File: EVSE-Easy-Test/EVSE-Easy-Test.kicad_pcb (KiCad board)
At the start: 2 copper layers, 70.1 x 40.9 mm, 17 parts, among them J1 Type 2, J2 CP diag, SW1 PP current, SW2 CP state

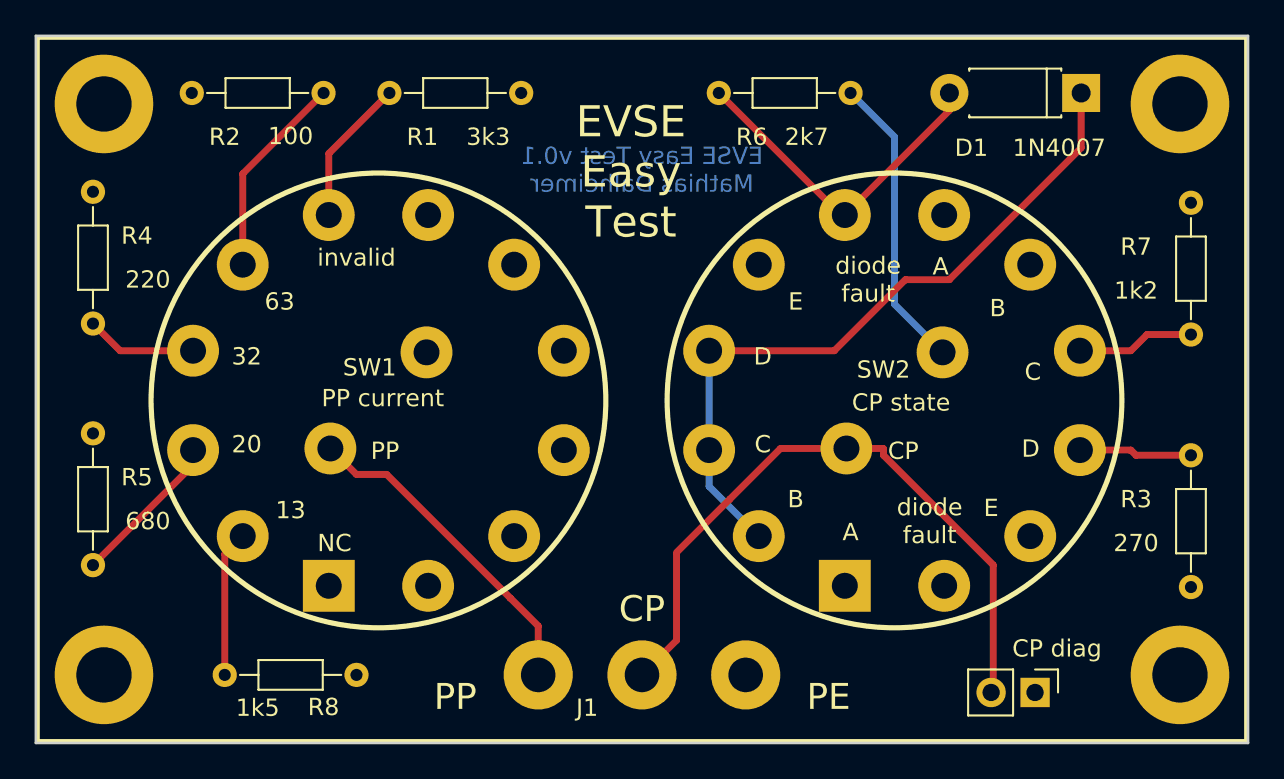
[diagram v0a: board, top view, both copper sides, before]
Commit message: second prototype as ordered
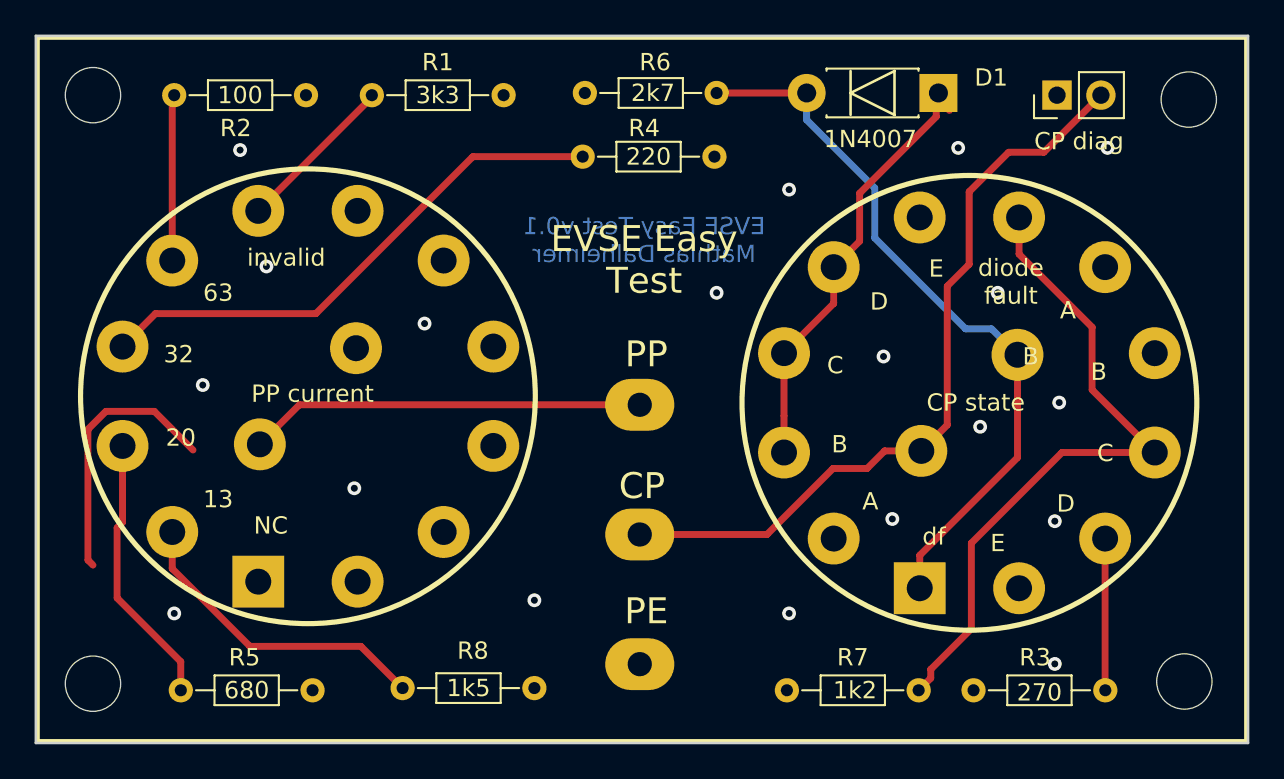
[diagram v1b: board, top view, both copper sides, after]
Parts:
- removed the REF** at (106.7, 44.5)
- removed the REF** at (44.5, 44.5)
- removed the REF** at (44.5, 77.5)
- removed the REF** at (106.7, 77.5)
- added REF**: MountingHole_3.2mm_M3, Mounting_Holes:MountingHole_3.2mm_M3, F.Cu at (107.2, 44.2)
- added REF**: MountingHole_3.2mm_M3, Mounting_Holes:MountingHole_3.2mm_M3, F.Cu at (43.8, 78.0)
- added REF**: MountingHole_3.2mm_M3, Mounting_Holes:MountingHole_3.2mm_M3, F.Cu at (43.8, 43.9)
- added REF**: MountingHole_3.2mm_M3, Mounting_Holes:MountingHole_3.2mm_M3, F.Cu at (106.9, 77.9)
- D1: footprint Diodes_THT:D_DO-41_SOD81_P7.62mm_Horizontal -> local:D_DO-41_SOD81_P7.62mm_Horizontal
- J1: footprint local:Type2-Solderpads -> local:RIACon175_3poles_AKL175-03; moved to B.Cu
- J2: footprint Pin_Headers:Pin_Header_Straight_1x02_Pitch2.54mm -> local:Pin_Header_Straight_1x02_Pitch2.54mm
- R1, R2, R3, R4, R5, R6, R7, R8: footprint Resistors_THT:R_Axial_DIN0204_L3.6mm_D1.6mm_P7.62mm_Horizontal -> local:R_Axial_DIN0204_L3.6mm_D1.6mm_P7.62mm_Horizontal
- moved R7 36.6 mm to (83.9, 78.4), turned to 0 degrees
- moved R4 36.0 mm to (79.8, 47.5), turned to 180 degrees
- moved J2 34.6 mm to (99.6, 43.9), turned to 90 degrees
- moved R5 19.5 mm to (56.5, 78.4), turned to 180 degrees
- moved R6 15.4 mm to (72.3, 43.8), turned to 0 degrees
- moved R3 13.9 mm to (94.7, 78.4), turned to 0 degrees
- moved R8 10.3 mm to (69.3, 78.2)
- moved D1 8.26 mm to (92.7, 43.8)
- moved J1 8.12 mm to (75.4, 69.3), turned to 90 degrees
- moved R2 6.61 mm to (56.1, 43.9), turned to 180 degrees
- moved SW2 4.33 mm to (94.5, 61.7)
- moved SW1 4.09 mm to (56.2, 61.4)
- moved R1 1.02 mm to (67.6, 43.9)
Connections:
- R6 pad 1: Net-(R6-Pad1) -> PE
- SW2 pad 1: (no net) -> Net-(D1-Pad2)
- SW2 pad 10: Net-(R3-Pad2) -> Net-(R7-Pad2)
- SW2 pad 11: (no net) -> Net-(R3-Pad2)
- SW2 pad 12: PE -> (no net)
- SW2 pad 14: Net-(R6-Pad1) -> Net-(D1-Pad2)
- SW2 pad 2: Net-(D1-Pad1) -> (no net)
- SW2 pad 5: PE -> Net-(D1-Pad1)
- SW2 pad 6: Net-(D1-Pad2) -> PE
- SW2 pad 7: (no net) -> Net-(R7-Pad2)
- SW2 pad 8: PE -> (no net)
- SW2 pad 9: Net-(R7-Pad2) -> (no net)
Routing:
- net Net-(R7-Pad2): track 6.81 -> 39.4 mm
- net Net-(R4-Pad2): track 6.44 -> 31.2 mm
- net Net-(D1-Pad2): track 19.8 -> 42.1 mm
- net Net-(R6-Pad1): track 17.2 -> 0.00 mm
- net Net-(D1-Pad1): track 41.5 -> 25.6 mm
- net PE: track 0.00 -> 15.4 mm, vias 0 -> 19
- net Net-(R8-Pad2): track 8.46 -> 18.3 mm
- net Net-(R5-Pad2): track 9.05 -> 15.8 mm
- net CP: track 39.1 -> 44.4 mm
- net PP: track 19.1 -> 22.9 mm
- net Net-(R2-Pad2): track 11.9 -> 9.61 mm
- net Net-(R3-Pad2): track 6.55 -> 8.78 mm
- net Net-(R1-Pad2): track 8.51 -> 9.41 mm
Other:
- board text added: "df"
